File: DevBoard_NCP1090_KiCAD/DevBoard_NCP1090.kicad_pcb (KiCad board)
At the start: 2 copper layers, 22.2 x 21.6 mm, 12 parts, among them U1 NCP1090, X1 Conn_01x04, X2 Conn_01x03

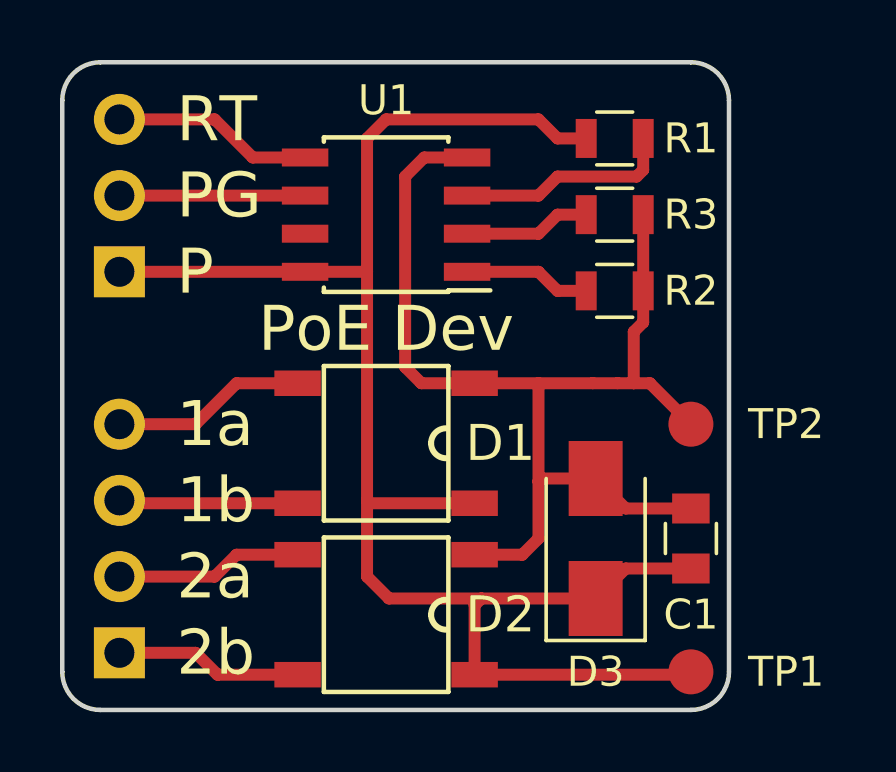
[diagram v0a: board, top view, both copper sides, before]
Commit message: v2 initial commit
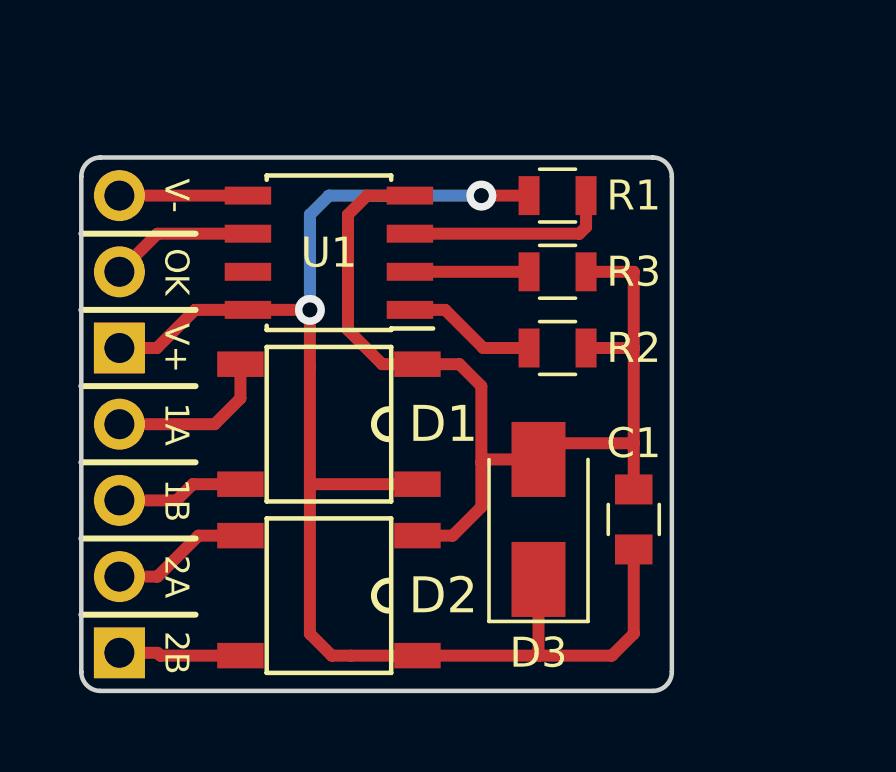
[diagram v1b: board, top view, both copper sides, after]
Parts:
- removed TP1, TP2: MountingHole_Pad, Measurement_Points:Measurement_Point_Round-SMD-Pad_Small
- moved R1 2.69 mm to (108.6, 91.4)
- moved R2 2.69 mm to (108.6, 96.5)
- moved R3 2.69 mm to (108.6, 94.0)
- moved X2 2.54 mm to (94.0, 96.5)
- moved U1 2.29 mm to (101.0, 93.3)
- moved C1 2.01 mm to (111.1, 102.2)
- moved D3 2.01 mm to (108.0, 102.2)
- moved D1 2.01 mm to (101.0, 99.1)
- moved D2 2.01 mm to (101.0, 104.8)
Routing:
- net /P: track 55.7 -> 48.8 mm, vias 0 -> 2
- net /N: track 37.8 -> 33.7 mm
- net /RTN: track 6.72 -> 4.28 mm
- net /BR2b: track 6.24 -> 4.07 mm
- net /BR2a: track 6.24 -> 4.60 mm
- net /BR1b: track 5.98 -> 4.39 mm
- net /PGOOD: track 6.19 -> 4.81 mm
- net /BR1a: track 6.51 -> 5.53 mm
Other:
- board size 22.2 x 21.6 mm -> 19.7 x 17.8 mm
- net class Default: via_dia 0.8 -> 1; via_drill 0.4 -> 0.5
- board text added: "1A"
- board text added: "1B"
- board text added: "2A"
- board text added: "2B"
- board text added: "NCP1090 802.3af PoE Development Board Designed by Alex M. Version 2"
- board text added: "OK"
- board text added: "V+"
- board text added: "V-"
- board text removed: "1a"
- board text removed: "1b"
- board text removed: "2a"
- board text removed: "2b"
- board text removed: "NCP1090 802.3af PoE Development Board Designed by Alex M. Version 1"
- board text removed: "P"
- board text removed: "PG"
- board text removed: "PoE Dev"
- board text removed: "RT"
